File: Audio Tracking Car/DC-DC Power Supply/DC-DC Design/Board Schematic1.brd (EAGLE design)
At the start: 160 x 100 mm, 24 parts, among them IC1 TL081P, IC2 LM393N, Q1 BSS295

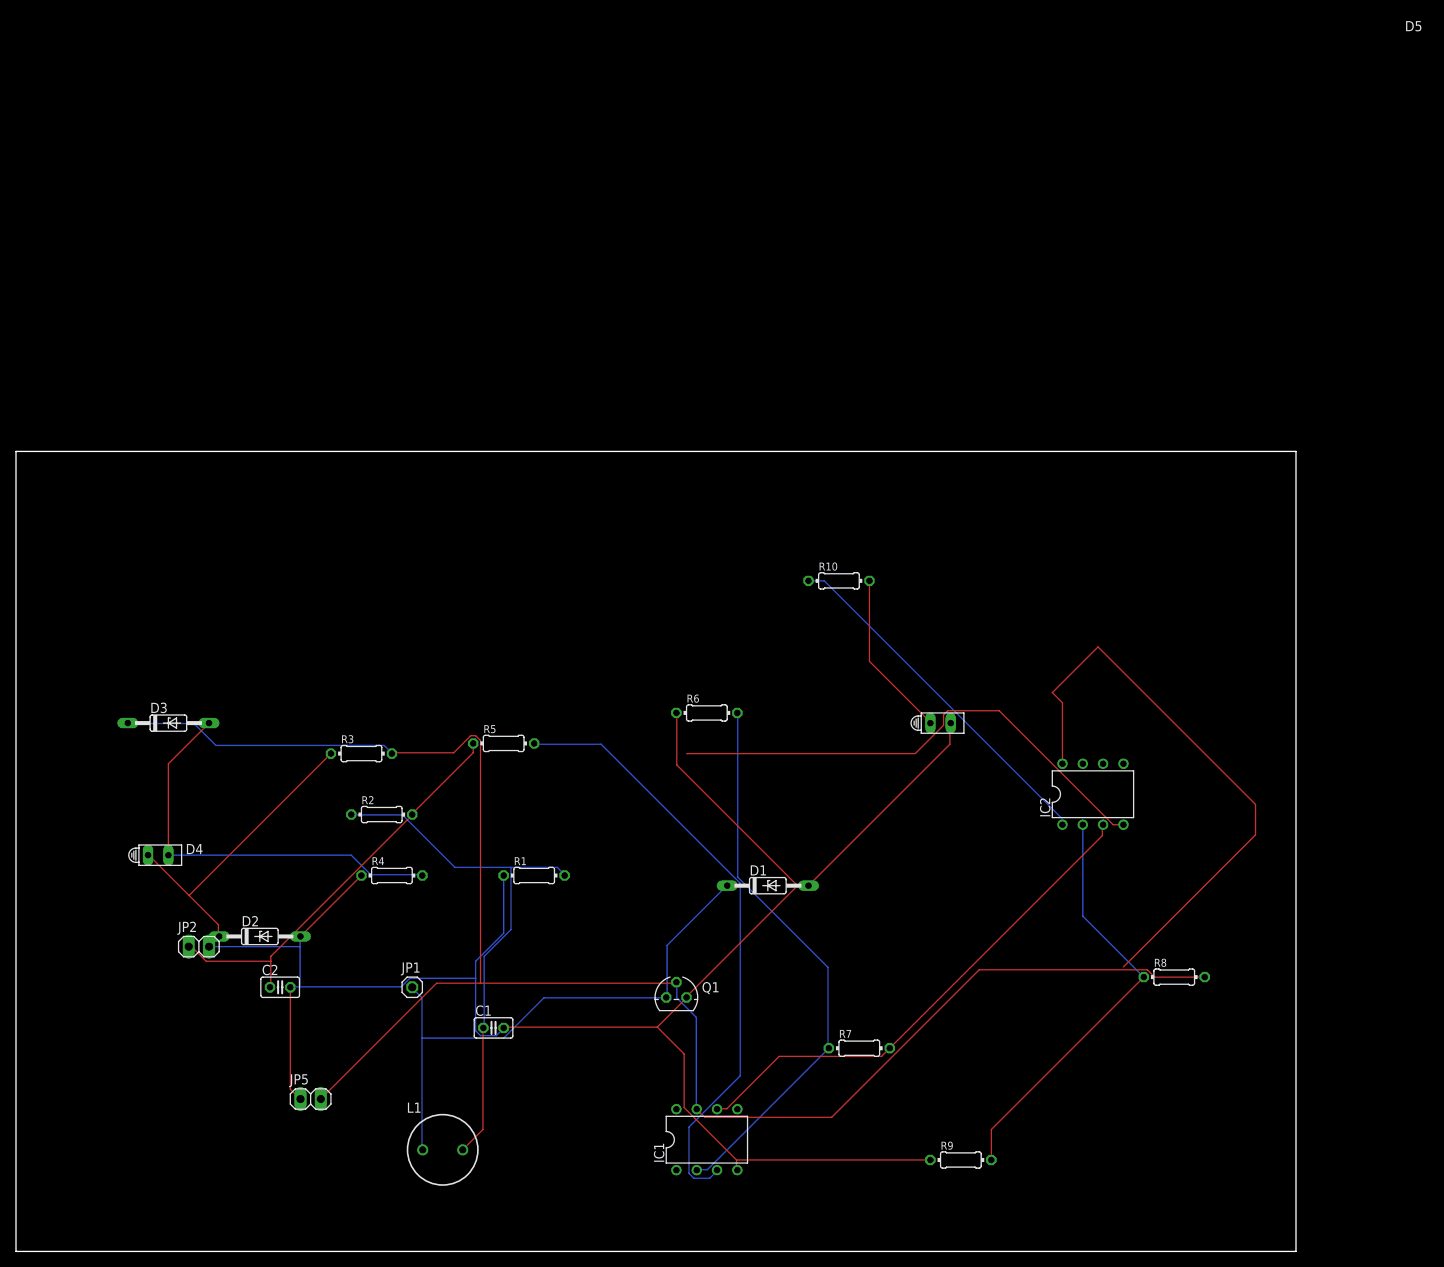
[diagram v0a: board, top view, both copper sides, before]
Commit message: new new
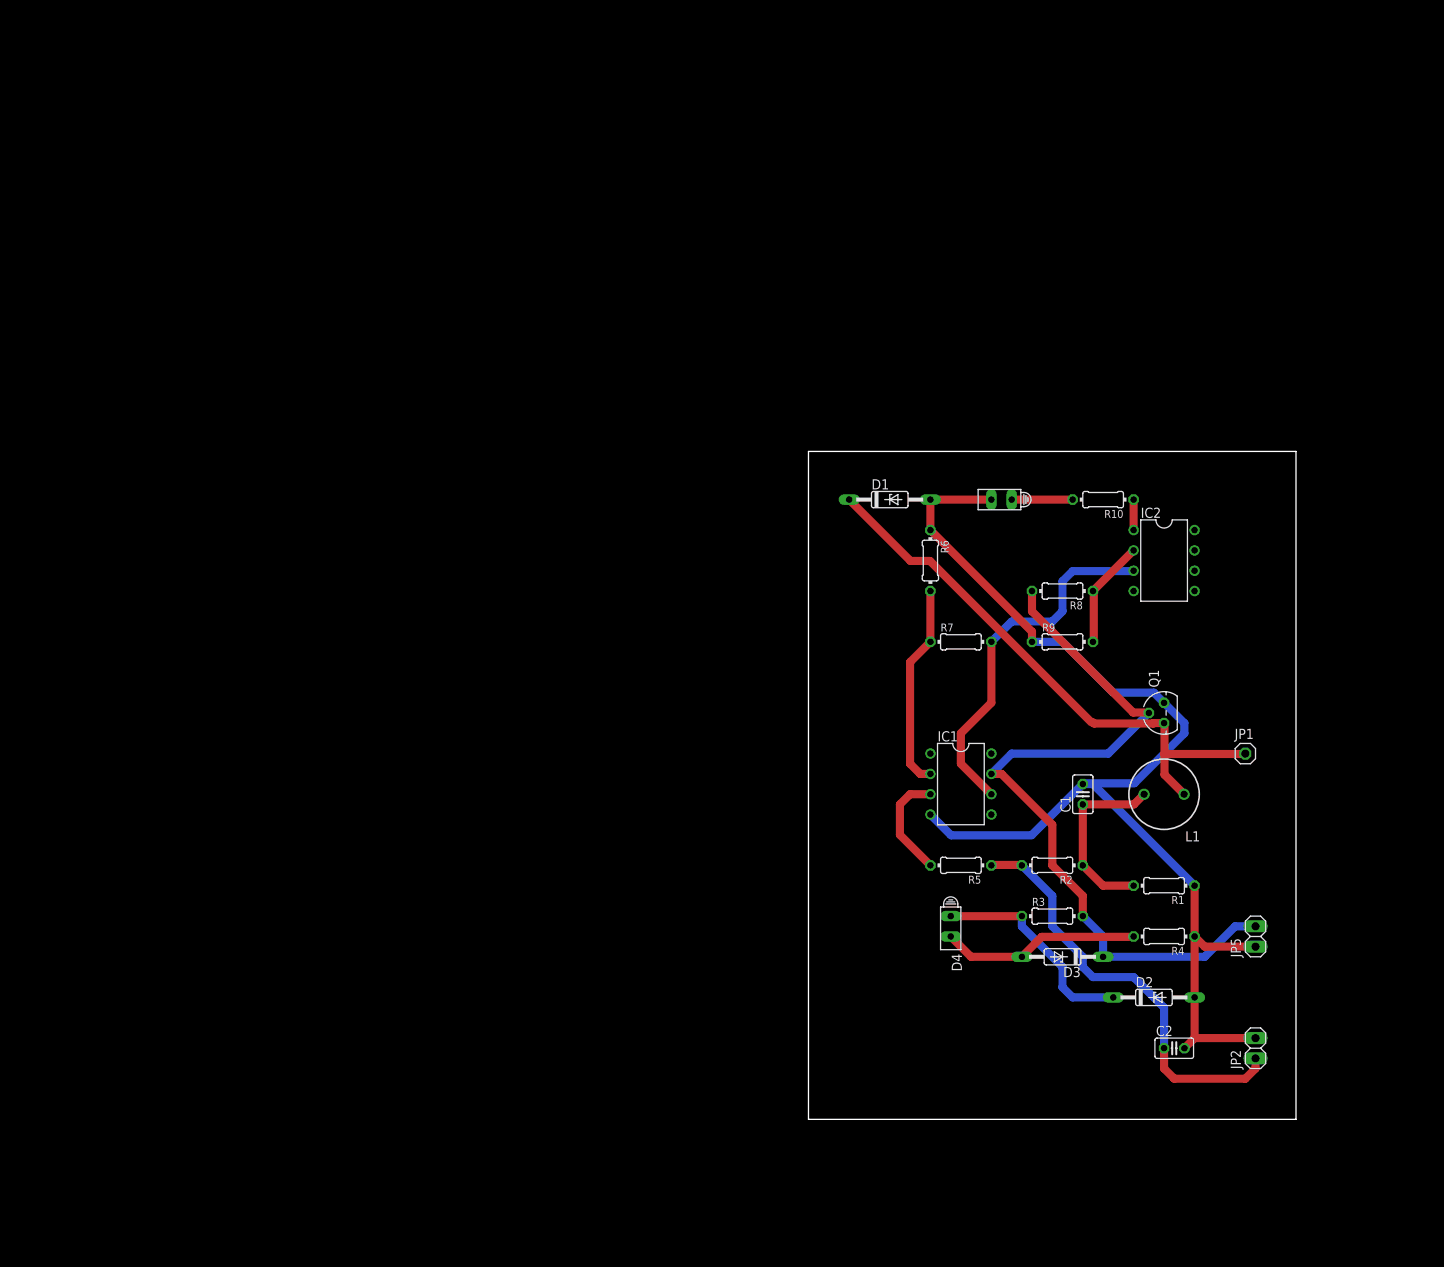
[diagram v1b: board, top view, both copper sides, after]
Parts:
- moved JP2 132.7 mm to (154.9, 25.4), turned to 90 degrees
- moved JP5 119.8 mm to (154.9, 39.4), turned to 90 degrees
- moved D3 115.5 mm to (130.8, 36.8), turned to 180 degrees
- moved D2 112.0 mm to (142.2, 31.8)
- moved C2 112.0 mm to (144.8, 25.4)
- moved JP1 108.2 mm to (153.7, 62.2)
- moved L1 100.5 mm to (143.5, 57.1), turned to 180 degrees
- moved D4 99.5 mm to (116.8, 40.6), turned to 270 degrees
- moved R4 96.8 mm to (143.5, 39.4), turned to 180 degrees
- moved R3 88.7 mm to (129.5, 41.9)
- moved R2 84.1 mm to (129.5, 48.3), turned to 180 degrees
- moved C1 79.2 mm to (133.3, 57.1), turned to 90 degrees
- moved R1 78.8 mm to (143.5, 45.7), turned to 180 degrees
- moved Q1 70.6 mm to (143.5, 67.3), turned to 90 degrees
- moved R9 66.0 mm to (130.8, 76.2)
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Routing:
- net N$1: track 216.6 -> 95.3 mm
- net V+: track 72.5 -> 0.00 mm
- net GND: track 239.2 -> 168.6 mm
- net V-: track 63.5 -> 0.00 mm
- net N$5: track 76.2 -> 13.5 mm
- net N$3: track 67.7 -> 23.2 mm
- net N$8: track 69.5 -> 25.7 mm
- net N$12: track 44.8 -> 3.81 mm
- net N$10: track 53.0 -> 13.8 mm
- net N$9: track 63.8 -> 45.9 mm
- net N$11: track 20.9 -> 7.62 mm
- net N$7: track 51.4 -> 38.5 mm
- net N$6: track 39.0 -> 26.8 mm
- net N$2: track 70.7 -> 77.1 mm
- net N$4: track 52.0 -> 53.4 mm
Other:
- board size 160 x 100 mm -> 60.9 x 83.5 mm
